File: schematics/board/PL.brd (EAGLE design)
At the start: 89 x 89 mm, 39 parts, among them IC2 STM32F103C8T, Q5 8MHz

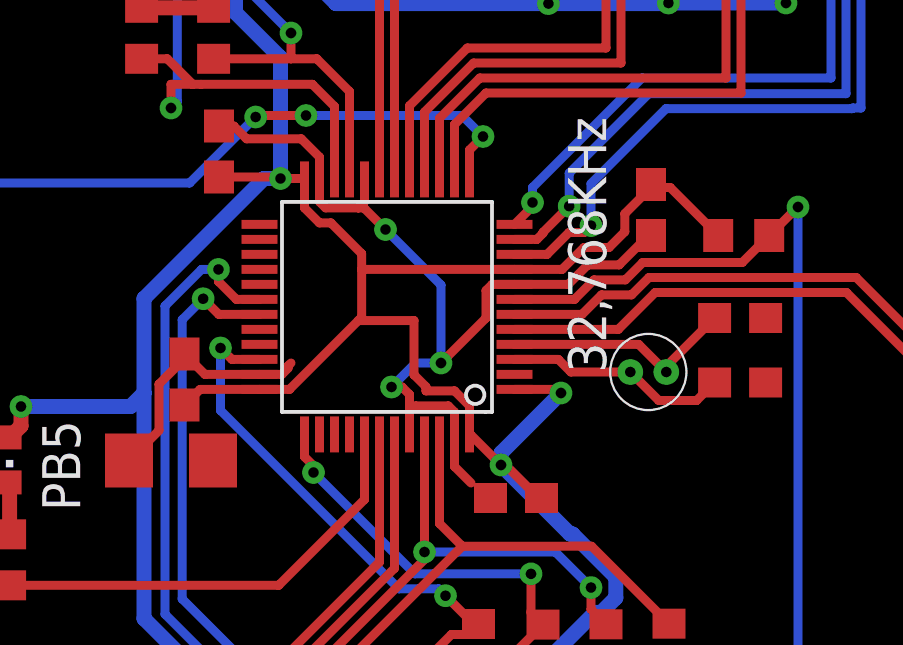
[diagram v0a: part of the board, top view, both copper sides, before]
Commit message: Обновлены герберы плат
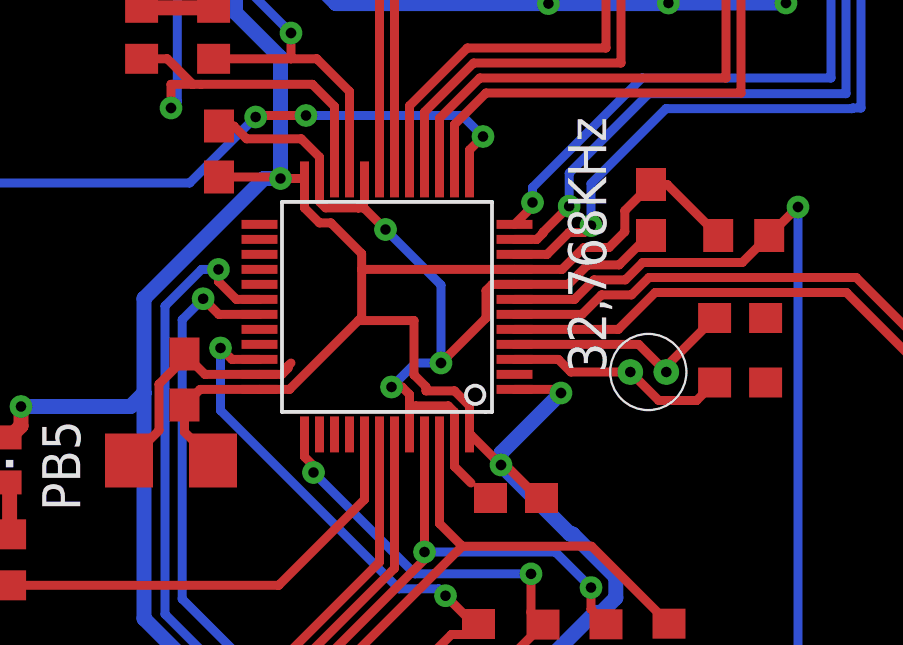
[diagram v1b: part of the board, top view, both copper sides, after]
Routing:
- net VDD: track 262.9 -> 265.3 mm
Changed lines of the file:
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@@
 <param name="mvStopFrame" value="1"/>
 <param name="mvCreamFrame" value="0"/>
-<param name="mlMinStopFrame" value="4mil"/>
-<param name="mlMaxStopFrame" value="4mil"/>
+<param name="mlMinStopFrame" value="2mil"/>
+<param name="mlMaxStopFrame" value="2mil"/>
 <param name="mlMinCreamFrame" value="0mil"/>
 <param name="mlMaxCreamFrame" value="0mil"/>
@@
 <wire x1="55.95" y1="32.5720875" x2="55.95" y2="31.62" width="0.3" layer="1"/>
 <wire x1="48.95" y1="33.12" x2="49.95" y2="33.12" width="0.3" layer="1"/>
-<wire x1="64.24" y1="38.25" x2="62.64" y2="39.85" width="0.3" layer="1"/>
 <via x="49.65" y="40.15" extent="1-16" drill="0.35"/>
-<wire x1="62" y1="39.85" x2="62.64" y2="39.85" width="0.3" layer="1"/>
 <wire x1="45.1" y1="25.47966875" x2="51.6532" y2="18.92646875" width="0.5" layer="16"/>
 <wire x1="45.1" y1="25.47966875" x2="45.1" y2="33" width="0.5" layer="16"/>
@@
 <wire x1="57.15" y1="30.6" x2="57" y2="30.6" width="0.3" layer="1"/>
 <wire x1="60.60163125" y1="37.85" x2="61.1282" y2="38.37656875" width="0.3" layer="1"/>
-<wire x1="61.1282" y1="38.37656875" x2="61.1282" y2="38.9782" width="0.3" layer="1"/>
-<wire x1="61.1282" y1="38.9782" x2="62" y2="39.85" width="0.3" layer="1"/>
 <wire x1="59.035775" y1="37.12" x2="59.765775" y2="37.85" width="0.3" layer="1"/>
 <wire x1="59.765775" y1="37.85" x2="60.60163125" y2="37.85" width="0.3" layer="1"/>
 <wire x1="57.45" y1="37.12" x2="59.035775" y2="37.12" width="0.3" layer="1"/>
-<wire x1="62" y1="39.85" x2="62" y2="39.95" width="0" layer="19" extent="1-1"/>
-<wire x1="47.4" y1="30.75" x2="46.45" y2="32.6" width="0" layer="19" extent="1-1"/>
+<wire x1="61.1282" y1="39.0782" x2="62" y2="39.95" width="0.3" layer="1"/>
+<wire x1="61.1282" y1="38.37656875" x2="61.1282" y2="39.0782" width="0.3" layer="1"/>
+<wire x1="62" y1="39.95" x2="62.54" y2="39.95" width="0.3" layer="1"/>
+<wire x1="62.54" y1="39.95" x2="64.24" y2="38.25" width="0.3" layer="1"/>
+<wire x1="46.45" y1="32.6" x2="46.45" y2="31.7" width="0.3" layer="1"/>
+<wire x1="46.45" y1="31.7" x2="47.4" y2="30.75" width="0.3" layer="1"/>
 </signal>
 <signal name="N$133">
